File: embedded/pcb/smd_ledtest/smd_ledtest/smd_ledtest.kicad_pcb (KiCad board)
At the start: 2 copper layers, 25.4 x 24.4 mm, 14 parts, among them J1 USB_C_Receptacle_USB2.0_16P

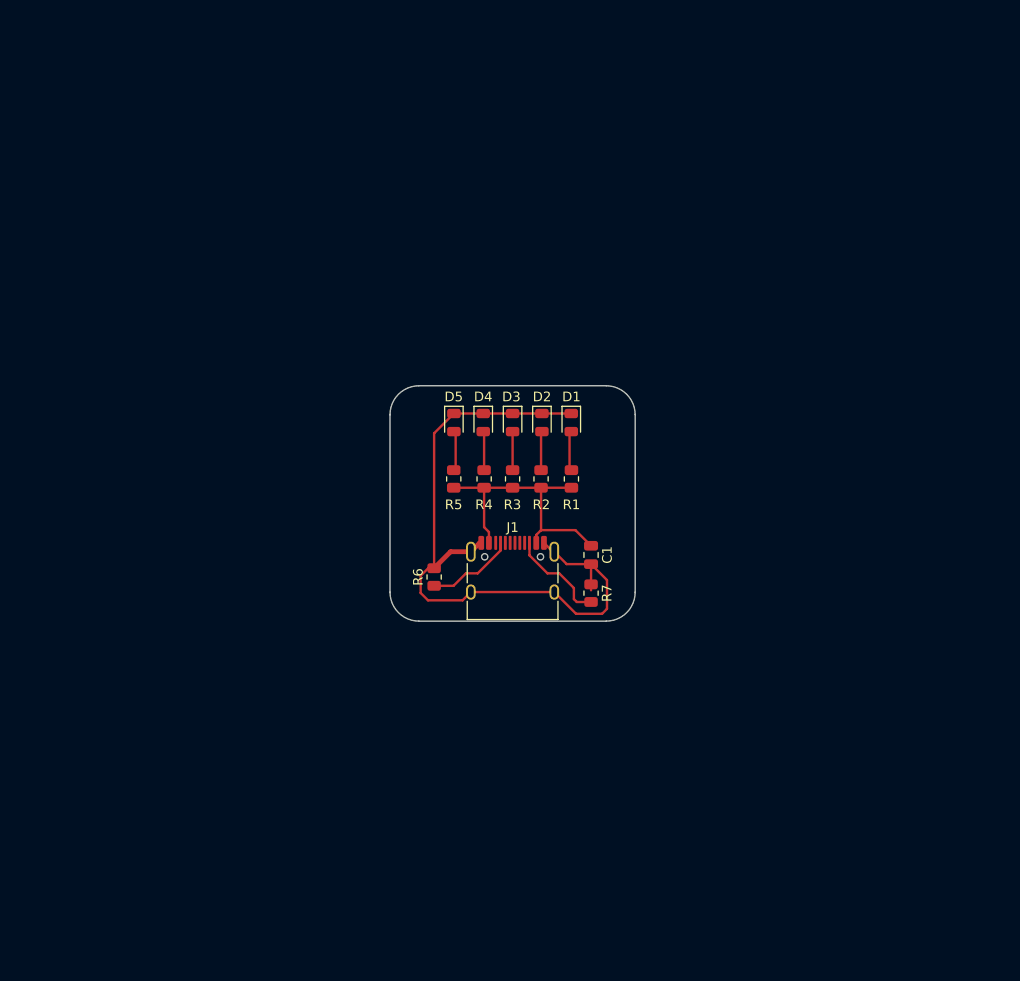
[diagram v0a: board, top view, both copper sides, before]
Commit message: added smd_led practice pcb
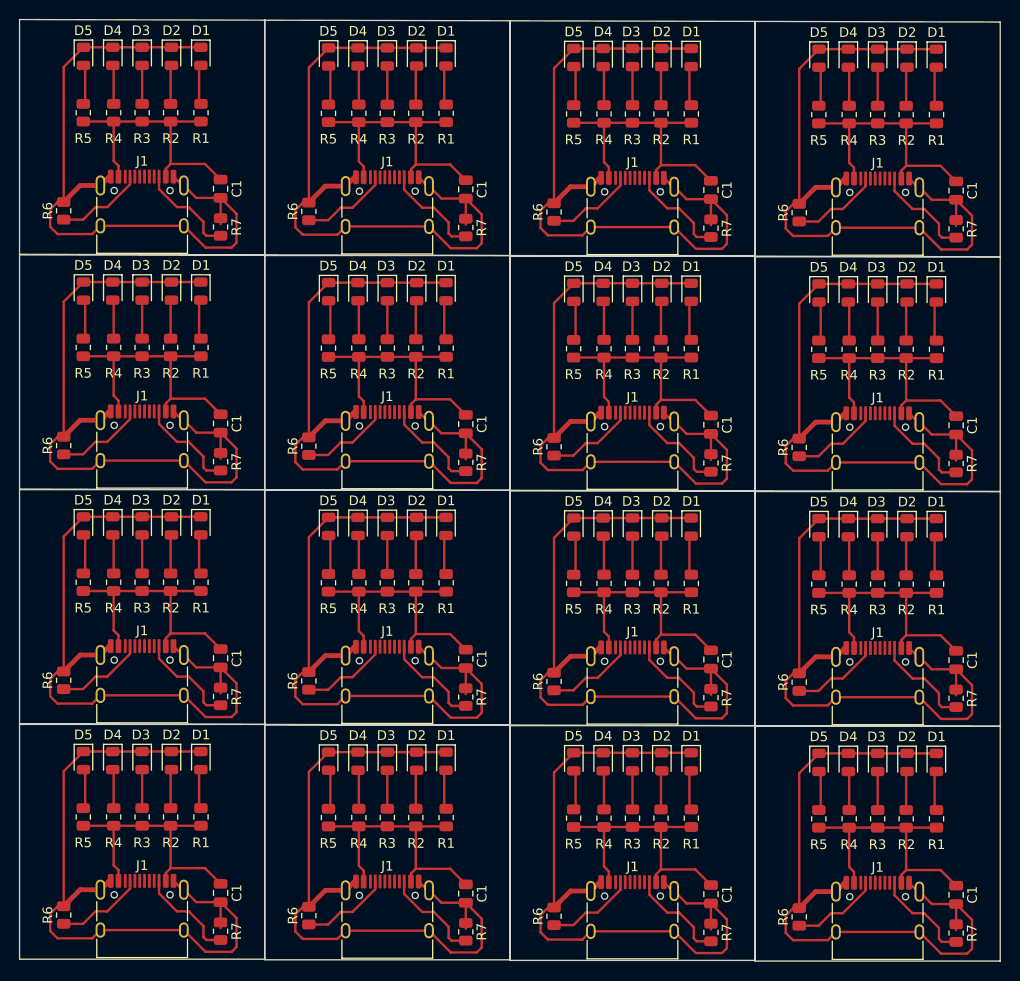
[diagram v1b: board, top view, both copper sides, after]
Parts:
- added C1: 10uF, Capacitor_SMD:C_0805_2012Metric, F.Cu at (111.2, 94.8)
- added C1: 10uF, Capacitor_SMD:C_0805_2012Metric, F.Cu at (111.2, 119.2)
- added C1: 10uF, Capacitor_SMD:C_0805_2012Metric, F.Cu at (162.0, 119.3)
- added C1: 10uF, Capacitor_SMD:C_0805_2012Metric, F.Cu at (136.6, 119.2)
- added C1: 10uF, Capacitor_SMD:C_0805_2012Metric, F.Cu at (136.6, 70.6)
- added C1: 10uF, Capacitor_SMD:C_0805_2012Metric, F.Cu at (162.0, 143.6)
- added C1: 10uF, Capacitor_SMD:C_0805_2012Metric, F.Cu at (187.4, 95.0)
- added C1: 10uF, Capacitor_SMD:C_0805_2012Metric, F.Cu at (136.6, 94.9)
- added C1: 10uF, Capacitor_SMD:C_0805_2012Metric, F.Cu at (187.4, 70.7)
- added C1: 10uF, Capacitor_SMD:C_0805_2012Metric, F.Cu at (162.0, 95.0)
- added C1: 10uF, Capacitor_SMD:C_0805_2012Metric, F.Cu at (187.4, 119.4)
- added C1: 10uF, Capacitor_SMD:C_0805_2012Metric, F.Cu at (111.2, 143.5)
- added C1: 10uF, Capacitor_SMD:C_0805_2012Metric, F.Cu at (136.6, 143.5)
- added C1: 10uF, Capacitor_SMD:C_0805_2012Metric, F.Cu at (162.0, 70.6)
- added C1: 10uF, Capacitor_SMD:C_0805_2012Metric, F.Cu at (187.4, 143.7)
- added D1: RED, LED_SMD:LED_0805_2012Metric, F.Cu at (134.6, 81.2)
- added D1: RED, LED_SMD:LED_0805_2012Metric, F.Cu at (160.0, 129.9)
- added D1: RED, LED_SMD:LED_0805_2012Metric, F.Cu at (109.2, 129.8)
- added D1: RED, LED_SMD:LED_0805_2012Metric, F.Cu at (134.6, 105.5)
- added D1: RED, LED_SMD:LED_0805_2012Metric, F.Cu at (109.2, 105.4)
- added D1: RED, LED_SMD:LED_0805_2012Metric, F.Cu at (160.0, 81.3)
- added D1: RED, LED_SMD:LED_0805_2012Metric, F.Cu at (134.6, 56.9)
- added D1: RED, LED_SMD:LED_0805_2012Metric, F.Cu at (185.4, 57.0)
- added D1: RED, LED_SMD:LED_0805_2012Metric, F.Cu at (134.6, 129.8)
- added D1: RED, LED_SMD:LED_0805_2012Metric, F.Cu at (185.4, 105.6)
- added D1: RED, LED_SMD:LED_0805_2012Metric, F.Cu at (109.2, 81.1)
- added D1: RED, LED_SMD:LED_0805_2012Metric, F.Cu at (160.0, 56.9)
- added D1: RED, LED_SMD:LED_0805_2012Metric, F.Cu at (185.4, 130.0)
- added D1: RED, LED_SMD:LED_0805_2012Metric, F.Cu at (160.0, 105.6)
- added D1: RED, LED_SMD:LED_0805_2012Metric, F.Cu at (185.4, 81.3)
- added D2: GREEN, LED_SMD:LED_0805_2012Metric, F.Cu at (131.5, 56.9)
- added D2: GREEN, LED_SMD:LED_0805_2012Metric, F.Cu at (156.9, 81.3)
- added D2: GREEN, LED_SMD:LED_0805_2012Metric, F.Cu at (182.3, 130.0)
- added D2: GREEN, LED_SMD:LED_0805_2012Metric, F.Cu at (131.5, 81.2)
- added D2: GREEN, LED_SMD:LED_0805_2012Metric, F.Cu at (156.9, 105.6)
- added D2: GREEN, LED_SMD:LED_0805_2012Metric, F.Cu at (131.5, 129.8)
- added D2: GREEN, LED_SMD:LED_0805_2012Metric, F.Cu at (131.5, 105.5)
- added D2: GREEN, LED_SMD:LED_0805_2012Metric, F.Cu at (182.3, 105.6)
- added D2: GREEN, LED_SMD:LED_0805_2012Metric, F.Cu at (106.1, 81.1)
- added D2: GREEN, LED_SMD:LED_0805_2012Metric, F.Cu at (182.3, 57.0)
- added D2: GREEN, LED_SMD:LED_0805_2012Metric, F.Cu at (106.1, 105.4)
- added D2: GREEN, LED_SMD:LED_0805_2012Metric, F.Cu at (106.1, 129.8)
- added D2: GREEN, LED_SMD:LED_0805_2012Metric, F.Cu at (156.9, 56.9)
- added D2: GREEN, LED_SMD:LED_0805_2012Metric, F.Cu at (156.9, 129.9)
- added D2: GREEN, LED_SMD:LED_0805_2012Metric, F.Cu at (182.3, 81.3)
- added D3: YELLOW, LED_SMD:LED_0805_2012Metric, F.Cu at (179.3, 81.3)
- added D3: YELLOW, LED_SMD:LED_0805_2012Metric, F.Cu at (179.3, 105.6)
- added D3: YELLOW, LED_SMD:LED_0805_2012Metric, F.Cu at (103.1, 129.8)
- added D3: YELLOW, LED_SMD:LED_0805_2012Metric, F.Cu at (128.5, 105.5)
- added D3: YELLOW, LED_SMD:LED_0805_2012Metric, F.Cu at (153.9, 81.3)
- added D3: YELLOW, LED_SMD:LED_0805_2012Metric, F.Cu at (179.3, 57.0)
- added D3: YELLOW, LED_SMD:LED_0805_2012Metric, F.Cu at (128.5, 81.2)
- added D3: YELLOW, LED_SMD:LED_0805_2012Metric, F.Cu at (179.3, 130.0)
- added D3: YELLOW, LED_SMD:LED_0805_2012Metric, F.Cu at (153.9, 105.6)
- added D3: YELLOW, LED_SMD:LED_0805_2012Metric, F.Cu at (153.9, 56.9)
- added D3: YELLOW, LED_SMD:LED_0805_2012Metric, F.Cu at (103.1, 105.4)
- added D3: YELLOW, LED_SMD:LED_0805_2012Metric, F.Cu at (153.9, 129.9)
- added D3: YELLOW, LED_SMD:LED_0805_2012Metric, F.Cu at (103.1, 81.1)
- added D3: YELLOW, LED_SMD:LED_0805_2012Metric, F.Cu at (128.5, 56.9)
- added D3: YELLOW, LED_SMD:LED_0805_2012Metric, F.Cu at (128.5, 129.8)
- added D4: BLUE, LED_SMD:LED_0805_2012Metric, F.Cu at (100.1, 81.1)
- added D4: BLUE, LED_SMD:LED_0805_2012Metric, F.Cu at (176.3, 57.0)
- added D4: BLUE, LED_SMD:LED_0805_2012Metric, F.Cu at (150.9, 129.9)
- added D4: BLUE, LED_SMD:LED_0805_2012Metric, F.Cu at (125.5, 81.2)
- added D4: BLUE, LED_SMD:LED_0805_2012Metric, F.Cu at (176.3, 105.6)
- added D4: BLUE, LED_SMD:LED_0805_2012Metric, F.Cu at (125.5, 129.8)
- added D4: BLUE, LED_SMD:LED_0805_2012Metric, F.Cu at (100.1, 105.4)
- added D4: BLUE, LED_SMD:LED_0805_2012Metric, F.Cu at (176.3, 130.0)
- added D4: BLUE, LED_SMD:LED_0805_2012Metric, F.Cu at (150.9, 105.6)
- added D4: BLUE, LED_SMD:LED_0805_2012Metric, F.Cu at (150.9, 81.3)
- added D4: BLUE, LED_SMD:LED_0805_2012Metric, F.Cu at (150.9, 56.9)
- added D4: BLUE, LED_SMD:LED_0805_2012Metric, F.Cu at (125.5, 56.9)
- added D4: BLUE, LED_SMD:LED_0805_2012Metric, F.Cu at (100.1, 129.8)
- added D4: BLUE, LED_SMD:LED_0805_2012Metric, F.Cu at (176.3, 81.3)
- added D4: BLUE, LED_SMD:LED_0805_2012Metric, F.Cu at (125.5, 105.5)
- added D5: WHITE, LED_SMD:LED_0805_2012Metric, F.Cu at (122.4, 56.9)
- added D5: WHITE, LED_SMD:LED_0805_2012Metric, F.Cu at (122.4, 81.2)
- added D5: WHITE, LED_SMD:LED_0805_2012Metric, F.Cu at (97.0, 81.1)
- added D5: WHITE, LED_SMD:LED_0805_2012Metric, F.Cu at (147.8, 129.9)
- added D5: WHITE, LED_SMD:LED_0805_2012Metric, F.Cu at (173.2, 57.0)
- added D5: WHITE, LED_SMD:LED_0805_2012Metric, F.Cu at (173.2, 81.3)
- added D5: WHITE, LED_SMD:LED_0805_2012Metric, F.Cu at (173.2, 105.6)
- added D5: WHITE, LED_SMD:LED_0805_2012Metric, F.Cu at (97.0, 129.8)
- added D5: WHITE, LED_SMD:LED_0805_2012Metric, F.Cu at (122.4, 129.8)
- added D5: WHITE, LED_SMD:LED_0805_2012Metric, F.Cu at (147.8, 105.6)
- added D5: WHITE, LED_SMD:LED_0805_2012Metric, F.Cu at (147.8, 81.3)
- added D5: WHITE, LED_SMD:LED_0805_2012Metric, F.Cu at (97.0, 105.4)
- added D5: WHITE, LED_SMD:LED_0805_2012Metric, F.Cu at (173.2, 130.0)
- added D5: WHITE, LED_SMD:LED_0805_2012Metric, F.Cu at (122.4, 105.5)
- added D5: WHITE, LED_SMD:LED_0805_2012Metric, F.Cu at (147.8, 56.9)
- added J1: USB_C_Receptacle_USB2.0_16P, Connector_USB:USB_C_Receptacle_HRO_TYPE-C-31-M-12, F.Cu at (179.3, 146.5)
- added J1: USB_C_Receptacle_USB2.0_16P, Connector_USB:USB_C_Receptacle_HRO_TYPE-C-31-M-12, F.Cu at (128.5, 122.0)
- added J1: USB_C_Receptacle_USB2.0_16P, Connector_USB:USB_C_Receptacle_HRO_TYPE-C-31-M-12, F.Cu at (153.9, 122.1)
- added J1: USB_C_Receptacle_USB2.0_16P, Connector_USB:USB_C_Receptacle_HRO_TYPE-C-31-M-12, F.Cu at (128.5, 146.3)
- added J1: USB_C_Receptacle_USB2.0_16P, Connector_USB:USB_C_Receptacle_HRO_TYPE-C-31-M-12, F.Cu at (179.3, 97.8)
- added J1: USB_C_Receptacle_USB2.0_16P, Connector_USB:USB_C_Receptacle_HRO_TYPE-C-31-M-12, F.Cu at (103.1, 146.3)
- added J1: USB_C_Receptacle_USB2.0_16P, Connector_USB:USB_C_Receptacle_HRO_TYPE-C-31-M-12, F.Cu at (153.9, 73.4)
- added J1: USB_C_Receptacle_USB2.0_16P, Connector_USB:USB_C_Receptacle_HRO_TYPE-C-31-M-12, F.Cu at (179.3, 73.5)
- added J1: USB_C_Receptacle_USB2.0_16P, Connector_USB:USB_C_Receptacle_HRO_TYPE-C-31-M-12, F.Cu at (179.3, 122.1)
- added J1: USB_C_Receptacle_USB2.0_16P, Connector_USB:USB_C_Receptacle_HRO_TYPE-C-31-M-12, F.Cu at (128.5, 97.7)
- added J1: USB_C_Receptacle_USB2.0_16P, Connector_USB:USB_C_Receptacle_HRO_TYPE-C-31-M-12, F.Cu at (103.1, 122.0)
- added J1: USB_C_Receptacle_USB2.0_16P, Connector_USB:USB_C_Receptacle_HRO_TYPE-C-31-M-12, F.Cu at (153.9, 146.4)
- added J1: USB_C_Receptacle_USB2.0_16P, Connector_USB:USB_C_Receptacle_HRO_TYPE-C-31-M-12, F.Cu at (128.5, 73.4)
- added J1: USB_C_Receptacle_USB2.0_16P, Connector_USB:USB_C_Receptacle_HRO_TYPE-C-31-M-12, F.Cu at (103.1, 97.6)
- added J1: USB_C_Receptacle_USB2.0_16P, Connector_USB:USB_C_Receptacle_HRO_TYPE-C-31-M-12, F.Cu at (153.9, 97.8)
- added R1: 220, Resistor_SMD:R_0805_2012Metric, F.Cu at (134.6, 111.3)
- added R1: 220, Resistor_SMD:R_0805_2012Metric, F.Cu at (160.0, 62.8)
- added R1: 220, Resistor_SMD:R_0805_2012Metric, F.Cu at (109.2, 111.3)
- added R1: 220, Resistor_SMD:R_0805_2012Metric, F.Cu at (160.0, 87.1)
- added R1: 220, Resistor_SMD:R_0805_2012Metric, F.Cu at (160.0, 135.7)
- added R1: 220, Resistor_SMD:R_0805_2012Metric, F.Cu at (134.6, 62.7)
- added R1: 220, Resistor_SMD:R_0805_2012Metric, F.Cu at (185.4, 62.8)
- added R1: 220, Resistor_SMD:R_0805_2012Metric, F.Cu at (185.4, 135.8)
- added R1: 220, Resistor_SMD:R_0805_2012Metric, F.Cu at (160.0, 111.4)
- added R1: 220, Resistor_SMD:R_0805_2012Metric, F.Cu at (109.2, 87.0)
- added R1: 220, Resistor_SMD:R_0805_2012Metric, F.Cu at (185.4, 111.5)
- added R1: 220, Resistor_SMD:R_0805_2012Metric, F.Cu at (185.4, 87.2)
- added R1: 220, Resistor_SMD:R_0805_2012Metric, F.Cu at (134.6, 87.0)
- added R1: 220, Resistor_SMD:R_0805_2012Metric, F.Cu at (109.2, 135.6)
- added R1: 220, Resistor_SMD:R_0805_2012Metric, F.Cu at (134.6, 135.7)
- added R2: 220, Resistor_SMD:R_0805_2012Metric, F.Cu at (182.2, 135.8)
- added R2: 220, Resistor_SMD:R_0805_2012Metric, F.Cu at (106.0, 111.3)
- added R2: 220, Resistor_SMD:R_0805_2012Metric, F.Cu at (182.2, 87.2)
- added R2: 220, Resistor_SMD:R_0805_2012Metric, F.Cu at (131.4, 135.7)
- added R2: 220, Resistor_SMD:R_0805_2012Metric, F.Cu at (131.4, 62.7)
- added R2: 220, Resistor_SMD:R_0805_2012Metric, F.Cu at (106.0, 87.0)
- added R2: 220, Resistor_SMD:R_0805_2012Metric, F.Cu at (106.0, 135.6)
- added R2: 220, Resistor_SMD:R_0805_2012Metric, F.Cu at (156.8, 62.8)
- added R2: 220, Resistor_SMD:R_0805_2012Metric, F.Cu at (182.2, 111.5)
- added R2: 220, Resistor_SMD:R_0805_2012Metric, F.Cu at (156.8, 87.1)
- added R2: 220, Resistor_SMD:R_0805_2012Metric, F.Cu at (156.8, 135.7)
- added R2: 220, Resistor_SMD:R_0805_2012Metric, F.Cu at (156.8, 111.4)
- added R2: 220, Resistor_SMD:R_0805_2012Metric, F.Cu at (131.4, 111.3)
- added R2: 220, Resistor_SMD:R_0805_2012Metric, F.Cu at (182.2, 62.8)
- added R2: 220, Resistor_SMD:R_0805_2012Metric, F.Cu at (131.4, 87.0)
- added R3: 220, Resistor_SMD:R_0805_2012Metric, F.Cu at (153.9, 62.8)
- added R3: 220, Resistor_SMD:R_0805_2012Metric, F.Cu at (128.5, 62.7)
- added R3: 220, Resistor_SMD:R_0805_2012Metric, F.Cu at (179.3, 87.2)
- added R3: 220, Resistor_SMD:R_0805_2012Metric, F.Cu at (179.3, 111.5)
- added R3: 220, Resistor_SMD:R_0805_2012Metric, F.Cu at (153.9, 135.7)
- added R3: 220, Resistor_SMD:R_0805_2012Metric, F.Cu at (103.1, 135.6)
- added R3: 220, Resistor_SMD:R_0805_2012Metric, F.Cu at (128.5, 111.3)
- added R3: 220, Resistor_SMD:R_0805_2012Metric, F.Cu at (179.3, 62.8)
- added R3: 220, Resistor_SMD:R_0805_2012Metric, F.Cu at (153.9, 87.1)
- added R3: 220, Resistor_SMD:R_0805_2012Metric, F.Cu at (179.3, 135.8)
- added R3: 220, Resistor_SMD:R_0805_2012Metric, F.Cu at (103.1, 111.3)
- added R3: 220, Resistor_SMD:R_0805_2012Metric, F.Cu at (128.5, 135.7)
- added R3: 220, Resistor_SMD:R_0805_2012Metric, F.Cu at (128.5, 87.0)
- added R3: 220, Resistor_SMD:R_0805_2012Metric, F.Cu at (153.9, 111.4)
- added R3: 220, Resistor_SMD:R_0805_2012Metric, F.Cu at (103.1, 87.0)
- added R4: 220, Resistor_SMD:R_0805_2012Metric, F.Cu at (176.3, 135.8)
- added R4: 220, Resistor_SMD:R_0805_2012Metric, F.Cu at (125.5, 111.3)
- added R4: 220, Resistor_SMD:R_0805_2012Metric, F.Cu at (125.5, 87.0)
- added R4: 220, Resistor_SMD:R_0805_2012Metric, F.Cu at (176.3, 111.5)
- added R4: 220, Resistor_SMD:R_0805_2012Metric, F.Cu at (150.9, 62.8)
- added R4: 220, Resistor_SMD:R_0805_2012Metric, F.Cu at (100.2, 87.0)
- added R4: 220, Resistor_SMD:R_0805_2012Metric, F.Cu at (100.2, 111.3)
- added R4: 220, Resistor_SMD:R_0805_2012Metric, F.Cu at (176.3, 62.8)
- added R4: 220, Resistor_SMD:R_0805_2012Metric, F.Cu at (150.9, 87.1)
- added R4: 220, Resistor_SMD:R_0805_2012Metric, F.Cu at (125.5, 62.7)
- added R4: 220, Resistor_SMD:R_0805_2012Metric, F.Cu at (176.3, 87.2)
- added R4: 220, Resistor_SMD:R_0805_2012Metric, F.Cu at (150.9, 111.4)
- added R4: 220, Resistor_SMD:R_0805_2012Metric, F.Cu at (150.9, 135.7)
- added R4: 220, Resistor_SMD:R_0805_2012Metric, F.Cu at (125.5, 135.7)
- added R4: 220, Resistor_SMD:R_0805_2012Metric, F.Cu at (100.2, 135.6)
- added R5: 220, Resistor_SMD:R_0805_2012Metric, F.Cu at (173.2, 62.8)
- added R5: 220, Resistor_SMD:R_0805_2012Metric, F.Cu at (173.2, 111.5)
- added R5: 220, Resistor_SMD:R_0805_2012Metric, F.Cu at (147.8, 87.1)
- added R5: 220, Resistor_SMD:R_0805_2012Metric, F.Cu at (173.2, 87.2)
- added R5: 220, Resistor_SMD:R_0805_2012Metric, F.Cu at (97.0, 135.6)
- added R5: 220, Resistor_SMD:R_0805_2012Metric, F.Cu at (147.8, 62.8)
- added R5: 220, Resistor_SMD:R_0805_2012Metric, F.Cu at (173.2, 135.8)
- added R5: 220, Resistor_SMD:R_0805_2012Metric, F.Cu at (97.0, 111.3)
- added R5: 220, Resistor_SMD:R_0805_2012Metric, F.Cu at (147.8, 111.4)
- added R5: 220, Resistor_SMD:R_0805_2012Metric, F.Cu at (122.4, 62.7)
- added R5: 220, Resistor_SMD:R_0805_2012Metric, F.Cu at (122.4, 87.0)
- added R5: 220, Resistor_SMD:R_0805_2012Metric, F.Cu at (147.8, 135.7)
- added R5: 220, Resistor_SMD:R_0805_2012Metric, F.Cu at (122.4, 135.7)
- added R5: 220, Resistor_SMD:R_0805_2012Metric, F.Cu at (97.0, 87.0)
- added R5: 220, Resistor_SMD:R_0805_2012Metric, F.Cu at (122.4, 111.3)
- added R6: 5.1K, Resistor_SMD:R_0805_2012Metric, F.Cu at (145.8, 97.3)
- added R6: 5.1K, Resistor_SMD:R_0805_2012Metric, F.Cu at (145.8, 72.9)
- added R6: 5.1K, Resistor_SMD:R_0805_2012Metric, F.Cu at (120.4, 145.8)
- added R6: 5.1K, Resistor_SMD:R_0805_2012Metric, F.Cu at (120.4, 72.9)
- added R6: 5.1K, Resistor_SMD:R_0805_2012Metric, F.Cu at (95.0, 121.4)
- added R6: 5.1K, Resistor_SMD:R_0805_2012Metric, F.Cu at (120.4, 121.5)
- added R6: 5.1K, Resistor_SMD:R_0805_2012Metric, F.Cu at (171.2, 121.6)
- added R6: 5.1K, Resistor_SMD:R_0805_2012Metric, F.Cu at (95.0, 97.1)
- added R6: 5.1K, Resistor_SMD:R_0805_2012Metric, F.Cu at (145.8, 145.9)
- added R6: 5.1K, Resistor_SMD:R_0805_2012Metric, F.Cu at (95.0, 145.8)
- added R6: 5.1K, Resistor_SMD:R_0805_2012Metric, F.Cu at (145.8, 121.6)
- added R6: 5.1K, Resistor_SMD:R_0805_2012Metric, F.Cu at (120.4, 97.2)
- added R6: 5.1K, Resistor_SMD:R_0805_2012Metric, F.Cu at (171.2, 73.0)
- added R6: 5.1K, Resistor_SMD:R_0805_2012Metric, F.Cu at (171.2, 146.0)
- added R6: 5.1K, Resistor_SMD:R_0805_2012Metric, F.Cu at (171.2, 97.3)
- added R7: 5.1K, Resistor_SMD:R_0805_2012Metric, F.Cu at (187.4, 123.3)
- added R7: 5.1K, Resistor_SMD:R_0805_2012Metric, F.Cu at (187.4, 74.7)
- added R7: 5.1K, Resistor_SMD:R_0805_2012Metric, F.Cu at (111.2, 147.4)
- added R7: 5.1K, Resistor_SMD:R_0805_2012Metric, F.Cu at (136.6, 123.2)
- added R7: 5.1K, Resistor_SMD:R_0805_2012Metric, F.Cu at (187.4, 147.6)
- added R7: 5.1K, Resistor_SMD:R_0805_2012Metric, F.Cu at (136.6, 147.5)
- added R7: 5.1K, Resistor_SMD:R_0805_2012Metric, F.Cu at (111.2, 123.1)
- added R7: 5.1K, Resistor_SMD:R_0805_2012Metric, F.Cu at (162.0, 147.6)
- added R7: 5.1K, Resistor_SMD:R_0805_2012Metric, F.Cu at (136.6, 98.9)
- added R7: 5.1K, Resistor_SMD:R_0805_2012Metric, F.Cu at (187.4, 99.0)
- added R7: 5.1K, Resistor_SMD:R_0805_2012Metric, F.Cu at (162.0, 98.9)
- added R7: 5.1K, Resistor_SMD:R_0805_2012Metric, F.Cu at (162.0, 74.6)
- added R7: 5.1K, Resistor_SMD:R_0805_2012Metric, F.Cu at (136.6, 74.5)
- added R7: 5.1K, Resistor_SMD:R_0805_2012Metric, F.Cu at (162.0, 123.2)
- added R7: 5.1K, Resistor_SMD:R_0805_2012Metric, F.Cu at (111.2, 98.8)
- moved D2 54.0 mm to (106.1, 56.8)
- moved D3 54.0 mm to (103.1, 56.8)
- moved D5 54.0 mm to (97.0, 56.8)
- moved R1 54.0 mm to (109.2, 62.6)
- moved R2 54.0 mm to (106.0, 62.6)
- moved R3 54.0 mm to (103.1, 62.6)
- moved R5 54.0 mm to (97.0, 62.6)
- moved C1 54.0 mm to (111.2, 70.5)
- moved J1 54.0 mm to (103.1, 73.3)
- moved R6 54.0 mm to (95.0, 72.8)
- moved R7 54.0 mm to (111.2, 74.5)
- moved D1 54.0 mm to (109.2, 56.8)
- moved D4 54.0 mm to (100.1, 56.8)
- moved R4 54.0 mm to (100.2, 62.6)
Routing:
- net GND: track 73.4 -> 1175.0 mm
- net +5V: track 29.5 -> 471.7 mm
- net Net-(J1-CC2): track 10.3 -> 165.5 mm
- net Net-(J1-CC1): track 9.19 -> 147.0 mm
- net Net-(D5-A): track 4.07 -> 65.1 mm
- net Net-(D1-A): track 4.07 -> 65.1 mm
- net Net-(D2-A): track 4.03 -> 64.5 mm
- net Net-(D4-A): track 4.03 -> 64.5 mm
- net Net-(D3-A): track 3.99 -> 63.9 mm
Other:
- board size 25.4 x 24.4 mm -> 101.6 x 97.5 mm
